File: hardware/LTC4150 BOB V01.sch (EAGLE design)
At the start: 21 parts, among them U1 LTC4150

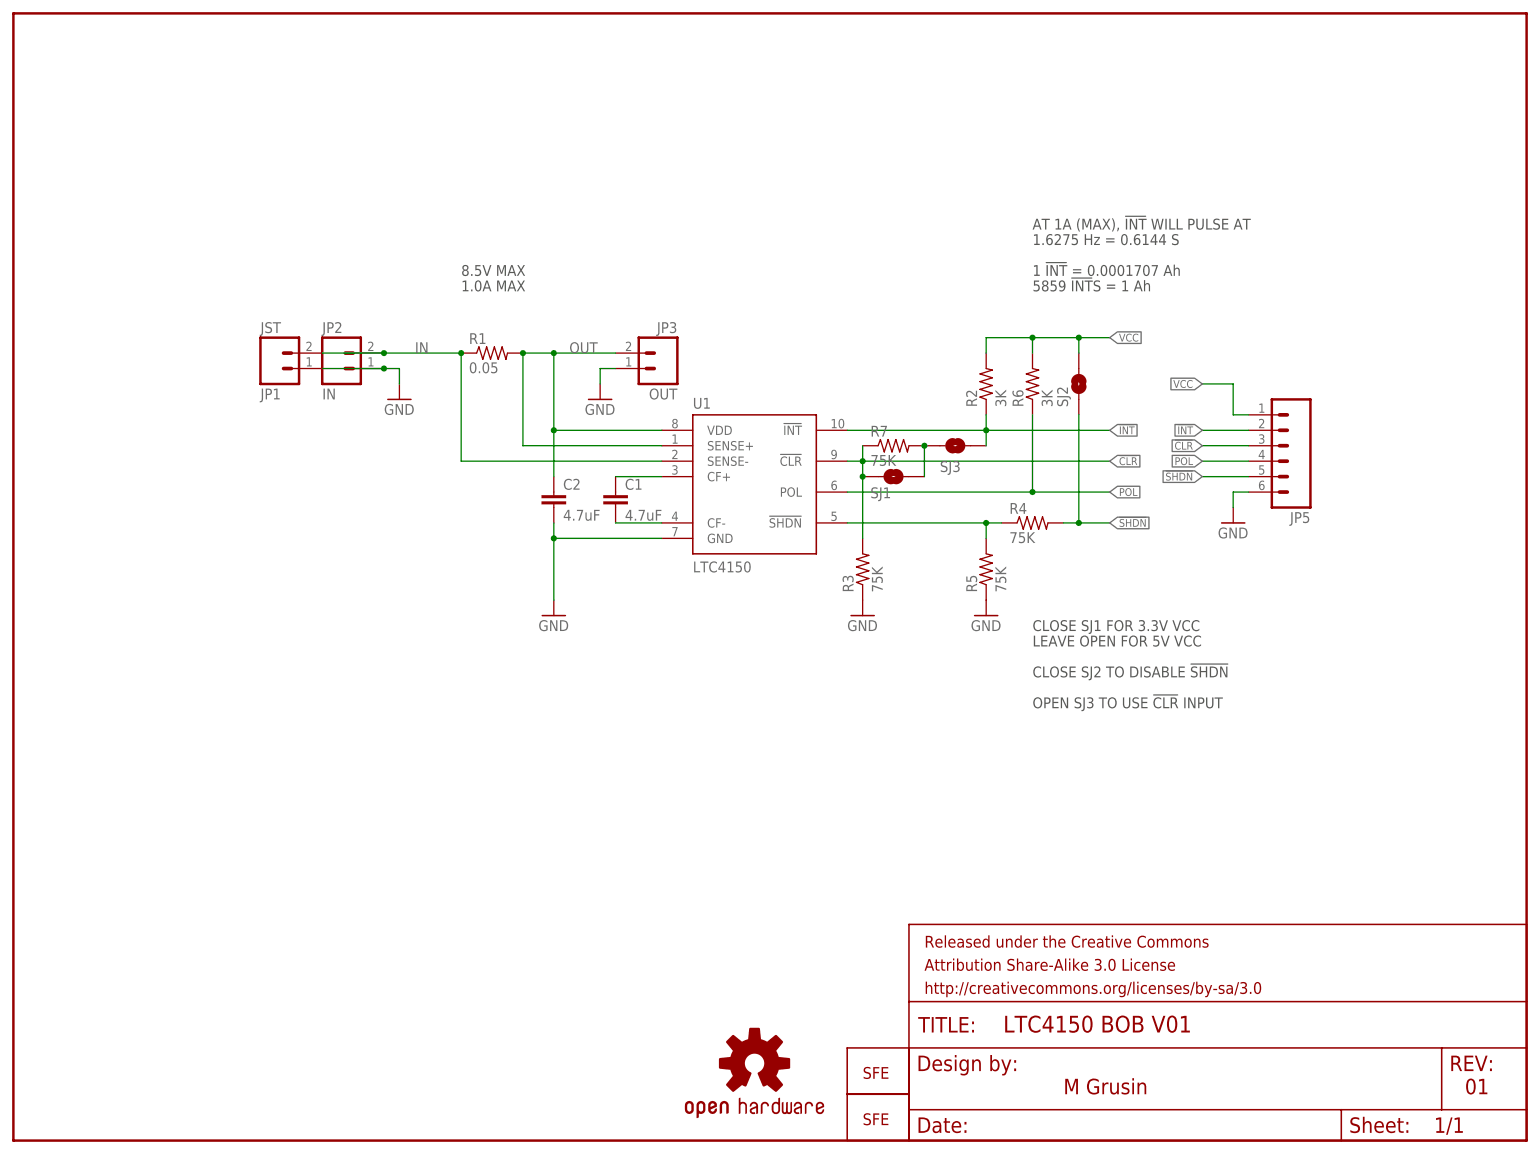
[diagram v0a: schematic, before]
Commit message: Ready for proto?
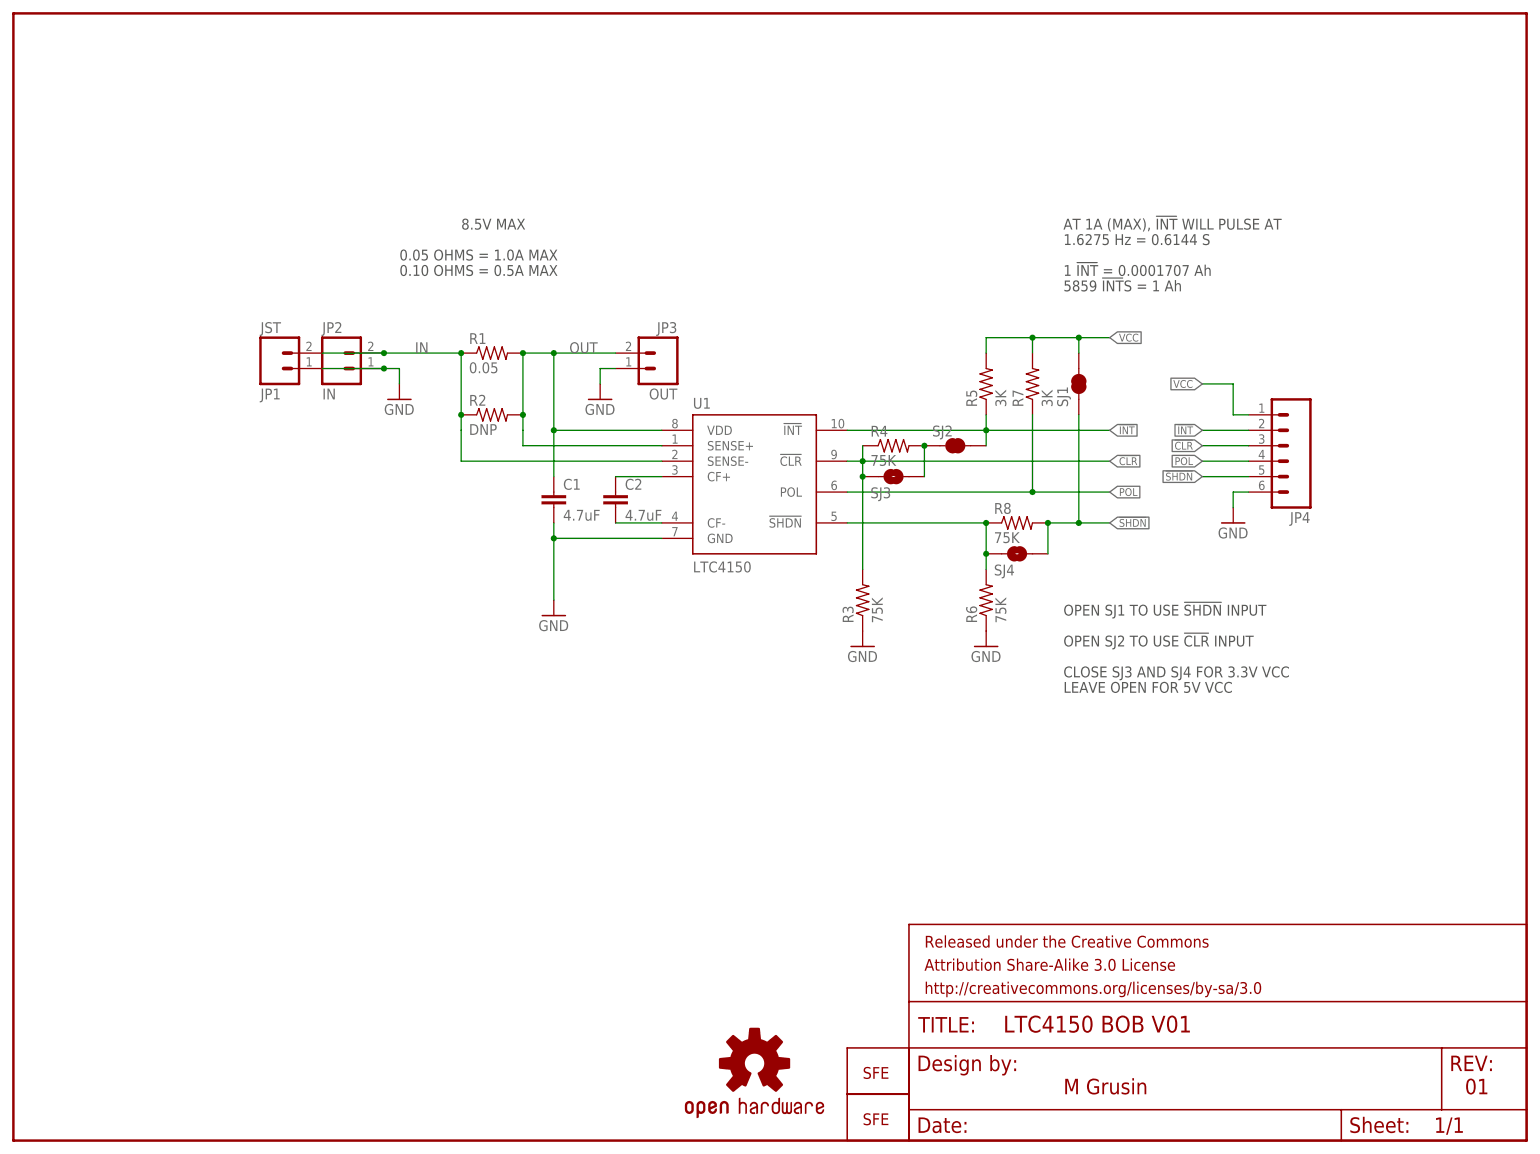
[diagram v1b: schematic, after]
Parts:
- added R8: 75K, SparkFun-Passives:RESISTOR0603-RES
- added SJ4: SOLDERJUMPERNO, mike-temp:SOLDERJUMPERNO
- LOGO1: value LOGO-SFESK -> OSHW-LOGOS; device SparkFun-Aesthetics:LOGO-SFESK -> SparkFun-Aesthetics:OSHW-LOGOS
- LOGO2: value OSHW-LOGOS -> LOGO-SFENW2; device SparkFun-Aesthetics:OSHW-LOGOS -> SparkFun-Aesthetics:LOGO-SFENW2
- LOGO3: value LOGO-SFENW2 -> LOGO-SFESK; device SparkFun-Aesthetics:LOGO-SFENW2 -> SparkFun-Aesthetics:LOGO-SFESK
- R2: value 3K -> DNP; device SparkFun-Passives:RESISTOR0603-RES -> SparkFun-Passives:RESISTORAXIAL-0.3
- R5, R7: value 75K -> 3K
- R6: value 3K -> 75K
- SJ1: value SOLDERJUMPERROUND -> SOLDERJUMPERNC; device mike-temp:SOLDERJUMPERROUND -> mike-temp:SOLDERJUMPERNC
- SJ2: value SOLDERJUMPERROUND -> SOLDERJUMPERNC; device mike-temp:SOLDERJUMPERROUND -> SparkFun-Passives:SOLDERJUMPERNC
- SJ3: value SOLDERJUMPERNC -> SOLDERJUMPERNO; device SparkFun-Passives:SOLDERJUMPERNC -> mike-temp:SOLDERJUMPERNO
- renumbered JP5 to JP4
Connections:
- net !CLR!: now also R4.1, SJ3.1; no longer R7.1, SJ1.1
- net !INT!: now also R5.1, SJ2.2; no longer R2.1, SJ3.2
- net !SHDN!: now also R8.2, SJ1.2, SJ4.2; no longer R4.2, SJ2.2
- net GND: now also C1.2, R6.1; no longer C2.2, R5.1
- net IN: now also R2.1
- net N$1: now also R4.2, SJ2.1, SJ3.2; no longer R7.2, SJ1.2, SJ3.1
- net N$3: now also C2.1; no longer C1.1
- net N$4: now also C2.2; no longer C1.2
- net N$9: now also R6.2, R8.1, SJ4.1; no longer R4.1, R5.2
- net OUT: now also C1.1, R2.2; no longer C2.1
- net POL: now also R7.1; no longer R6.1
- net VCC: now also R5.2, R7.2, SJ1.1; no longer R2.2, R6.2, SJ2.1
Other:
- note added: "0.05 OHMS = 1.0A MAX"
- note added: "0.10 OHMS = 0.5A MAX"
- note added: "CLOSE SJ3 AND SJ4 FOR 3.3V VCC"
- note added: "OPEN SJ1 TO USE !SHDN! INPUT"
- note added: "OPEN SJ2 TO USE !CLR! INPUT"
- note removed: "1.0A MAX"
- note removed: "CLOSE SJ1 FOR 3.3V VCC"
- note removed: "CLOSE SJ2 TO DISABLE !SHDN!"
- note removed: "OPEN SJ3 TO USE !CLR! INPUT"
- moved on the sheet: C1, C2, R2, R3, R4, R5, R6, R7, SJ1, SJ2, SJ3
